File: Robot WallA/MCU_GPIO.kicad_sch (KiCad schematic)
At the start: 2 parts, among them J13 10129383-916001ALF, J6 10129383-916001ALF

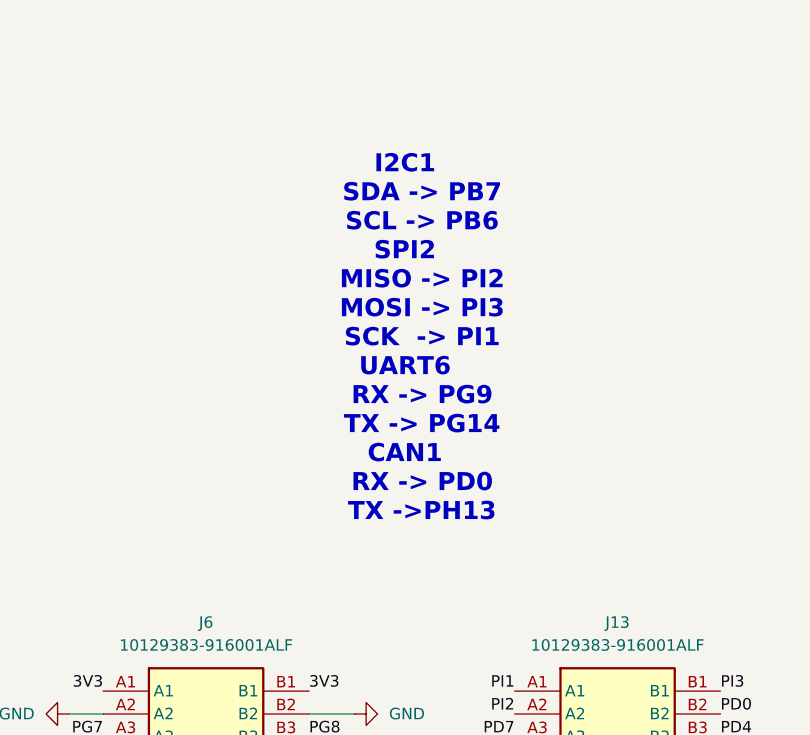
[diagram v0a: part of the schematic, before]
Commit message: Updated Fab files
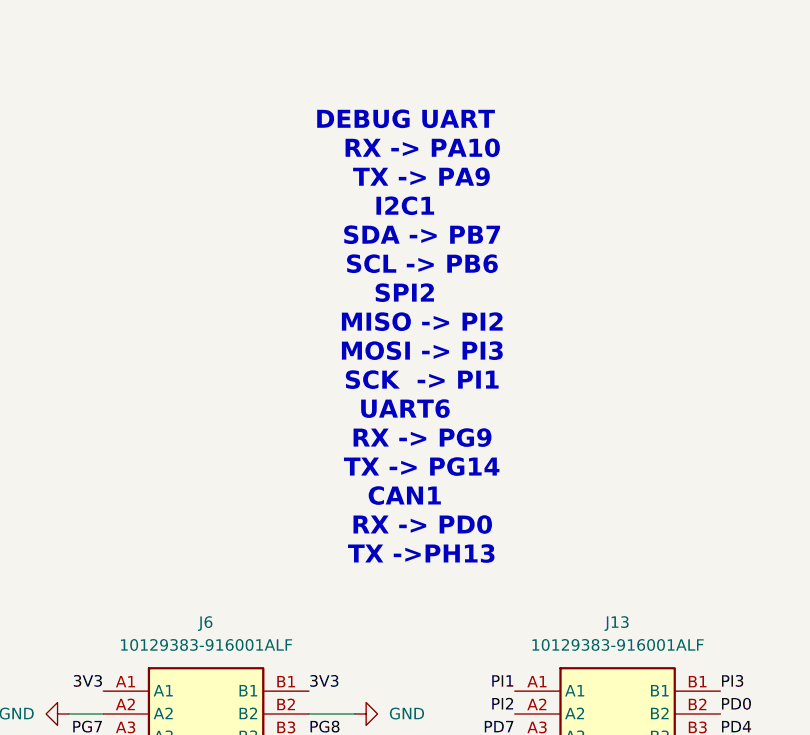
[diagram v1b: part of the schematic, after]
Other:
- note added: "DEBUG UART RX -> PA10 TX -> PA9 I2C1 SDA -> PB7 SCL -> PB6 SPI2 MISO -> PI2 MOSI -> PI3 SCK -> PI1 UART6 RX -> PG9 TX -> PG14 CAN1 RX -> PD0 TX ->PH13"
- note removed: "I2C1 SDA -> PB7 SCL -> PB6 SPI2 MISO -> PI2 MOSI -> PI3 SCK -> PI1 UART6 RX -> PG9 TX -> PG14 CAN1 RX -> PD0 TX ->PH13"
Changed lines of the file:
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@@
 		(comment 2 "THO")
 	)
-	(text "I2C1\n	SDA -> PB7\n	SCL -> PB6\nSPI2\n	MISO -> PI2\n	MOSI -> PI3\n	SCK  -> PI1\nUART6\n	RX -> PG9\n	TX -> PG14\nCAN1\n	RX -> PD0\n	TX ->PH13"
+	(text "DEBUG UART\n	RX -> PA10\n	TX -> PA9\nI2C1\n	SDA -> PB7\n	SCL -> PB6\nSPI2\n	MISO -> PI2\n	MOSI -> PI3\n	SCK  -> PI1\nUART6\n	RX -> PG9\n	TX -> PG14\nCAN1\n	RX -> PD0\n	TX ->PH13"
 		(exclude_from_sim no)
 		(at 100.838 51.054 0)
